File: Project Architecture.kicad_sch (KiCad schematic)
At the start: 0 parts

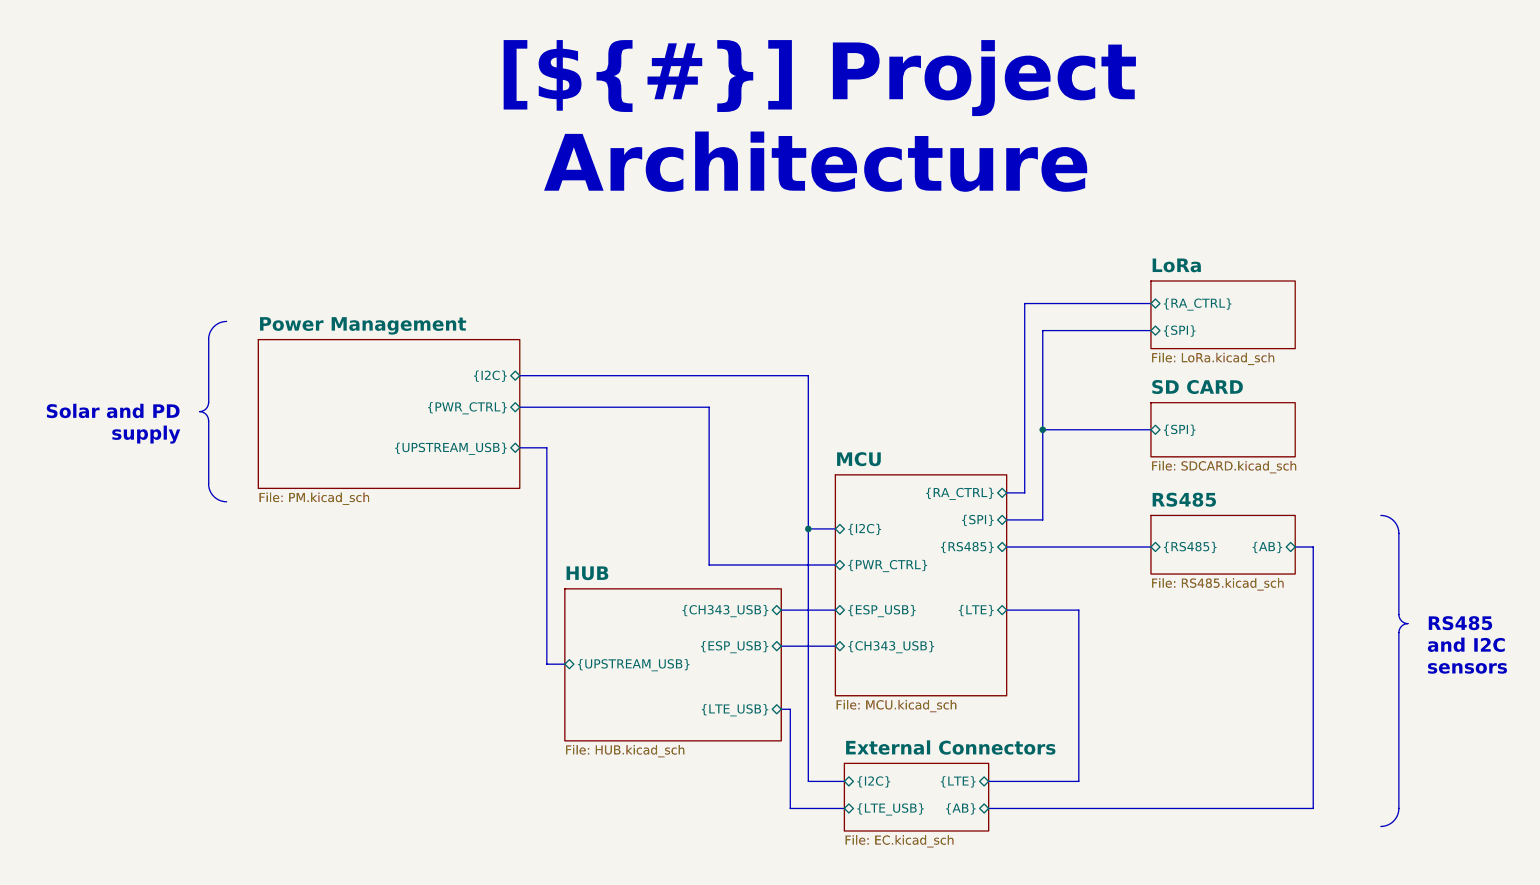
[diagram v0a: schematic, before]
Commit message: [PCB/SCH][Added] Preliminary version
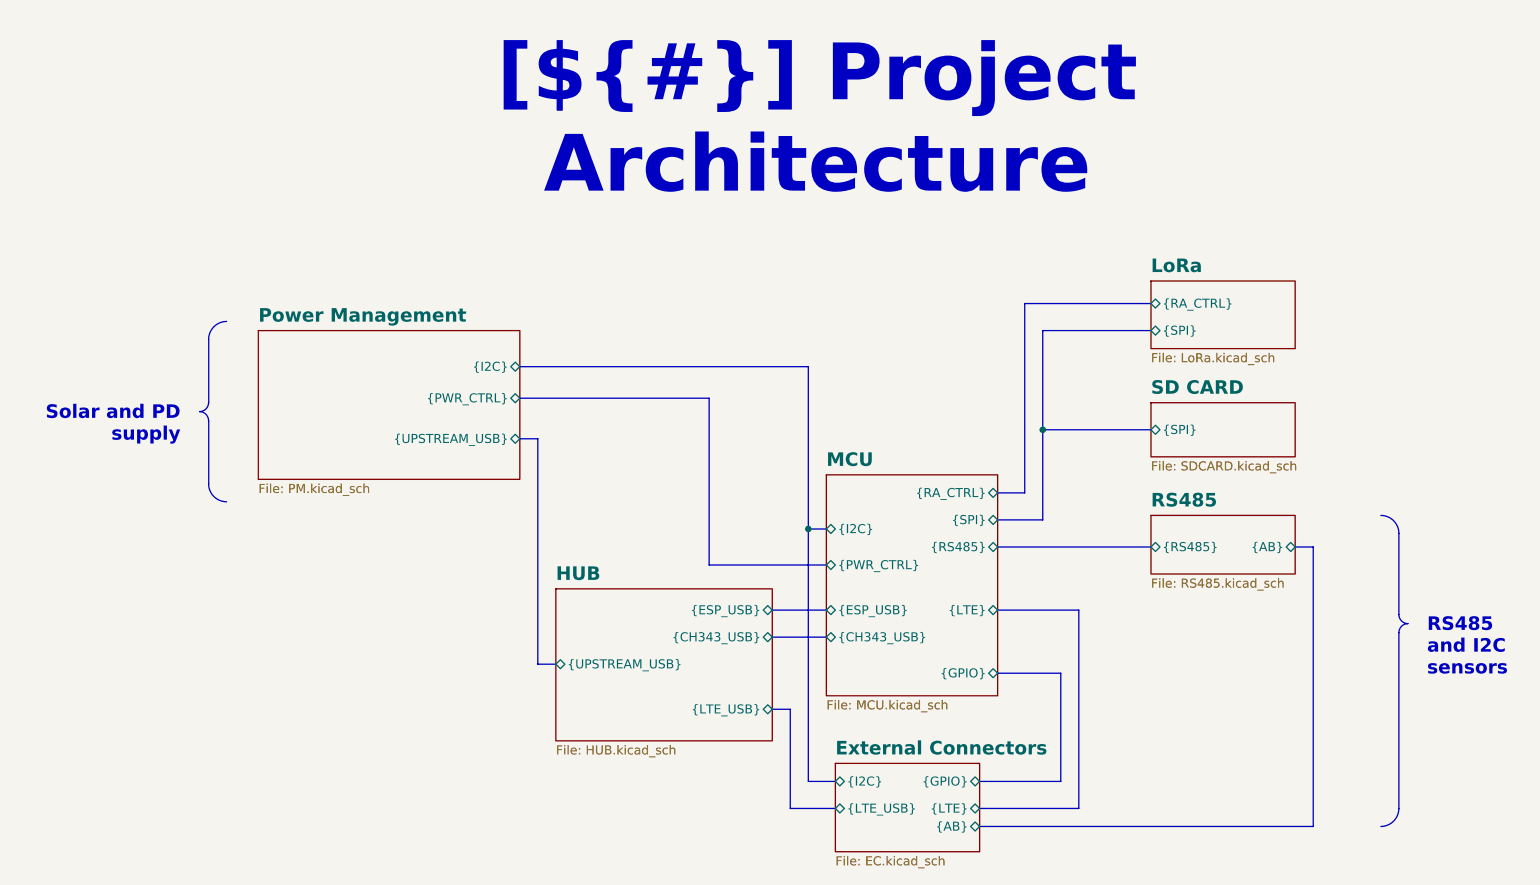
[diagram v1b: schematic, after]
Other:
- sheet External Connectors ports: added {GPIO}; removed none
- sheet MCU ports: added {GPIO}; removed none
